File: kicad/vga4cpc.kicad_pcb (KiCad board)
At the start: 2 copper layers, 61.4 x 76.7 mm, 39 parts, among them J1 VGA socket, J2 CPC video port, SW1 VFreq sw, SW2 reset, U1 Pico

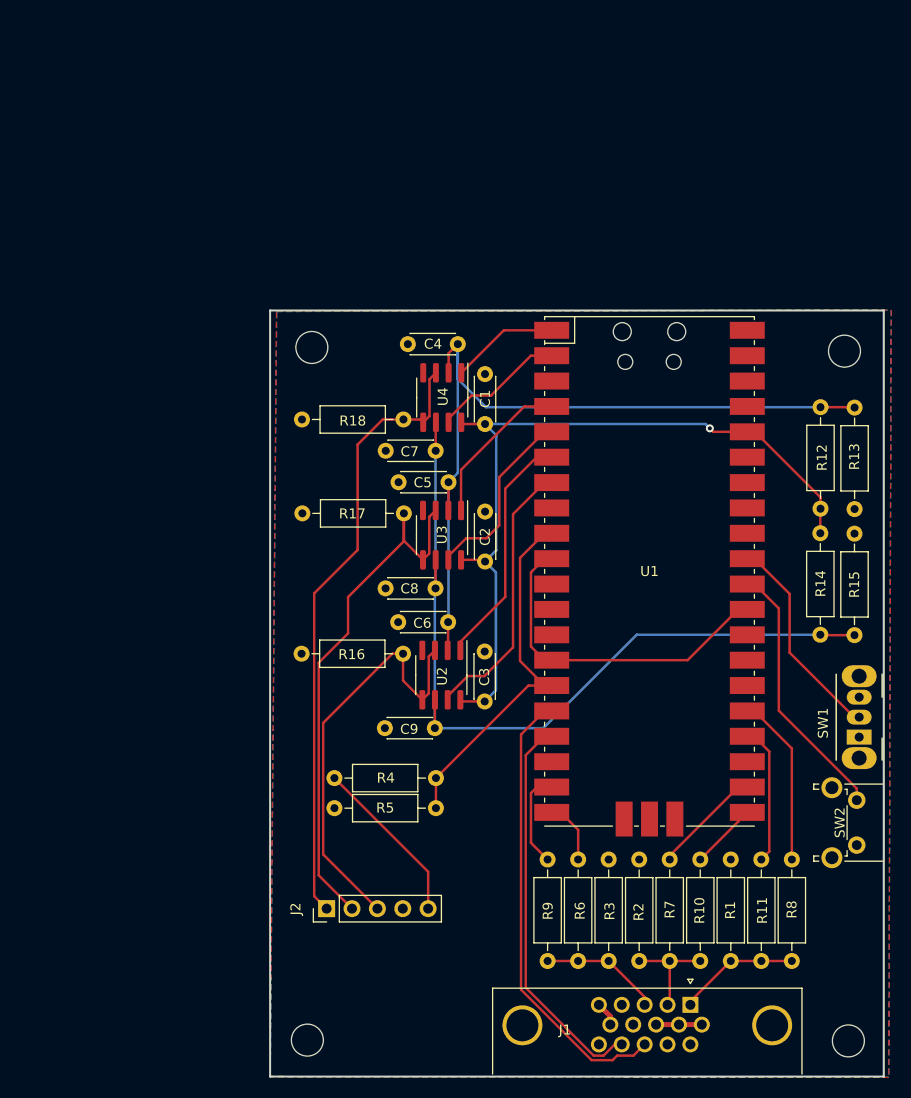
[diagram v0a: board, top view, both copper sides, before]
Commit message: Rotated
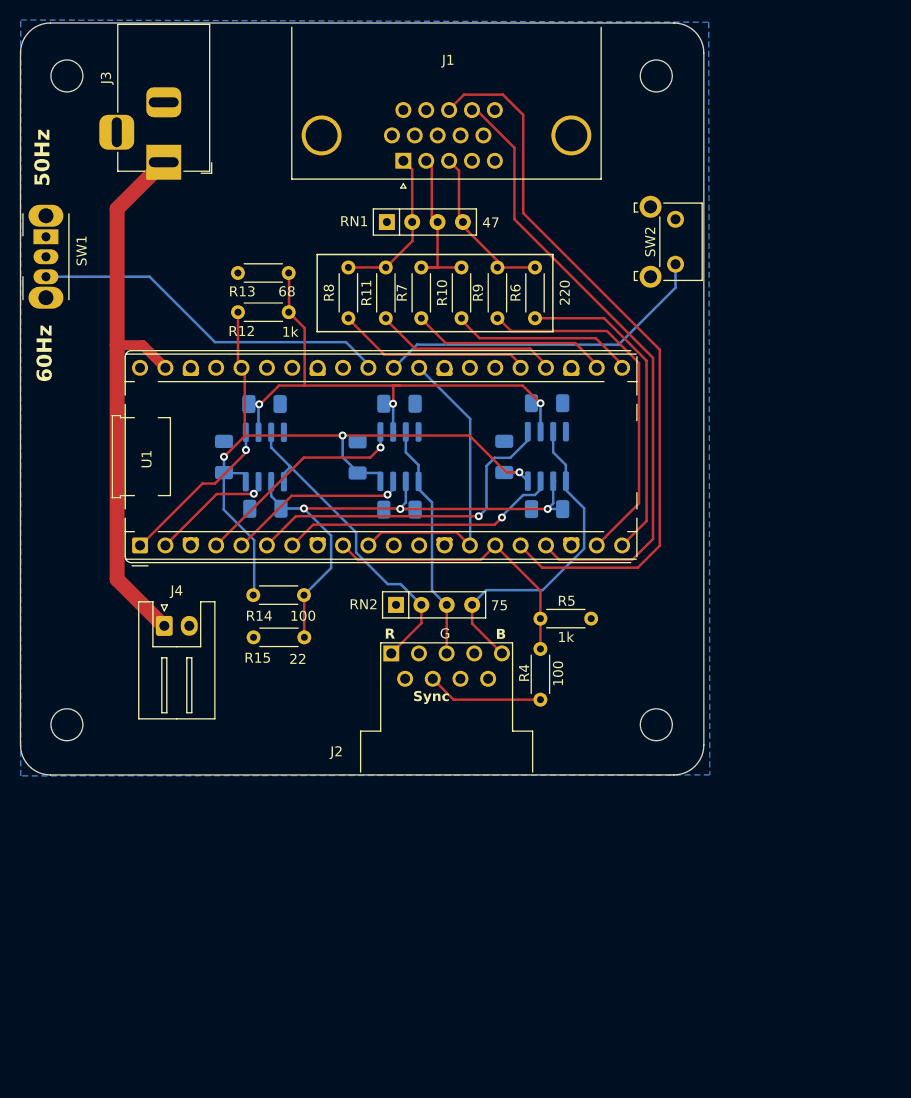
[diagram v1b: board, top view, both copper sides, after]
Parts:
- removed R1, R2, R3: 47, Resistor_THT:R_Axial_DIN0207_L6.3mm_D2.5mm_P10.16mm_Horizontal
- removed R16, R17, R18: 75, Resistor_THT:R_Axial_DIN0207_L6.3mm_D2.5mm_P10.16mm_Horizontal
- added J3: Barrel_Jack, Connector_BarrelJack:BarrelJack_Horizontal, F.Cu at (59.7, 36.6)
- added J4: Conn_01x02_Pin, Connector_JST:JST_XH_S2B-XH-A_1x02_P2.50mm_Horizontal, F.Cu at (59.8, 83.0)
- added RN1: 47, Resistor_THT:R_Array_SIP4, F.Cu at (82.0, 42.6)
- added RN2: 75, Resistor_THT:R_Array_SIP4, F.Cu at (82.9, 81.0)
- C1, C2, C3, C4, C5, C6, C7, C8, C9: footprint Capacitor_THT:C_Disc_D4.3mm_W1.9mm_P5.00mm -> Capacitor_SMD:C_1206_3216Metric_Pad1.33x1.80mm_HandSolder; moved to B.Cu
- J1: footprint Connector_Dsub:DSUB-15-HD_Female_Horizontal_P2.29x1.98mm_EdgePinOffset3.03mm_Housed_MountingHolesOffset4.94mm -> Connector_Dsub:DSUB-15-HD_Socket_Horizontal_P2.29x2.54mm_EdgePinOffset8.35mm_Housed_MountingHolesOffset10.89mm
- J2: value CPC video port -> DE9_Pins; footprint Connector_PinHeader_2.54mm:PinHeader_1x05_P2.54mm_Vertical -> Connector_Dsub:DSUB-9_Pins_Horizontal_P2.77x2.54mm_EdgePinOffset9.40mm
- R10, R11, R12, R13, R14, R4, R5, R6, R7, R8, R9: footprint Resistor_THT:R_Axial_DIN0207_L6.3mm_D2.5mm_P10.16mm_Horizontal -> Resistor_THT:R_Axial_DIN0204_L3.6mm_D1.6mm_P5.08mm_Horizontal
- R15: value 15 -> 22; footprint Resistor_THT:R_Axial_DIN0207_L6.3mm_D2.5mm_P10.16mm_Horizontal -> Resistor_THT:R_Axial_DIN0204_L3.6mm_D1.6mm_P5.08mm_Horizontal
- SW1: footprint Button_Switch_THT:SW_CuK_OS102011MA1QN1_SPDT_Angled -> Button_Switch_THT:SW_Slide_SPDT_Angled_CK_OS102011MA1Q
- SW2: footprint Button_Switch_THT:SW_Tactile_SPST_Angled_PTS645Vx31-2LFS -> Button_Switch_THT:SW_Tactile_SKHH_Angled
- U1: footprint pico:RPi_Pico_SMD_TH -> Pico:RaspberryPi_Pico_Common_THT_b
- U2, U3, U4: moved to B.Cu
- moved H1 102.6 mm to (109.0, 28.0), turned to 180 degrees
- moved SW1 95.6 mm to (47.9, 44.1), turned to -90 degrees
- moved J1 89.2 mm to (83.7, 36.5), turned to 180 degrees
- moved H2 82.6 mm to (50.0, 28.0), turned to 180 degrees
- moved R8 70.1 mm to (78.2, 52.3), turned to 90 degrees
- moved R11 65.9 mm to (81.9, 52.3), turned to 90 degrees
- moved R12 61.5 mm to (67.1, 51.6), turned to 0 degrees
- moved SW2 60.9 mm to (110.9, 42.4)
- moved R7 59.6 mm to (85.5, 52.3), turned to 90 degrees
- moved R10 59.2 mm to (89.5, 52.3), turned to 90 degrees
- moved R13 58.2 mm to (72.2, 47.7), turned to 180 degrees
- moved R14 57.1 mm to (68.7, 80.0), turned to 0 degrees
- moved R15 55.1 mm to (73.8, 84.2), turned to 180 degrees
- moved R9 54.4 mm to (93.1, 52.3), turned to 90 degrees
- moved R6 54.4 mm to (96.9, 52.3), turned to 90 degrees
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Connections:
- net 200mV renamed /Comparators/200mV
- net 430mV renamed /Comparators/600mV
- J2 pad 2: /Comparators/CPC_G -> GND
- J2 pad 3: /Comparators/CPC_R -> /Comparators/CPC_G
- J2 pad 5: /Connectors/CPC_CSYNC -> /Comparators/CPC_R
- SW1 pad 2: Net-(SW1-B) -> GND
- SW1 pad 3: GND -> Net-(SW1-C)
- SW2 pad 1: Net-(SW2-A) -> GND
- SW2 pad 2: GND -> Net-(SW2-B)
- U1 pad 30: Net-(SW2-A) -> Net-(SW2-B)
- U1 pad 31: Net-(SW1-B) -> Net-(SW1-C)
- U1 pad 39: unconnected-(U1-VSYS-Pad39) -> +5V
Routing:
- net +5V: track 0.00 -> 56.1 mm
- net Net-(SW1-C): track 0.00 -> 36.8 mm
- net Net-(SW2-B): track 0.00 -> 34.2 mm
- net /Comparators/CPC_G: track 55.4 -> 24.0 mm
- net /Comparators/CPC_B: track 62.0 -> 32.1 mm
- net /Connectors/VGA_HSYNC: track 44.8 -> 73.5 mm
- net Net-(U1-GPIO14): track 8.19 -> 36.1 mm
- net Net-(U1-GPIO15): track 5.44 -> 33.1 mm
- net /Comparators/600mV: track 82.0 -> 55.0 mm, vias 0 -> 3
- net Net-(SW2-A): track 25.9 -> 0.00 mm
- net /Connectors/VGA_VSYNC: track 38.8 -> 63.5 mm
- net /Comparators/200mV: track 81.4 -> 57.2 mm, vias 0 -> 3
- net Net-(SW1-B): track 20.0 -> 0.00 mm
- net Net-(U1-GPIO16): track 6.29 -> 18.8 mm
- net /Comparators/R0: track 22.5 -> 33.9 mm, vias 0 -> 1
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- removed copper zone on F.Cu, net GND
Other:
- board size 61.4 x 76.7 mm -> 68.4 x 75.3 mm
- board text added: "50Hz"
- board text added: "60Hz"
- board text added: "B"
- board text added: "G"
- board text added: "R"
- board text added: "R9"
- board text added: "Sync"
